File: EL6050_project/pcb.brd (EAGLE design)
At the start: 160 x 100 mm, 36 parts, among them IC1 MEGA8-P, IC2 MEGA8-P, X1 BU-SMA-V, X2 GMSTBA2

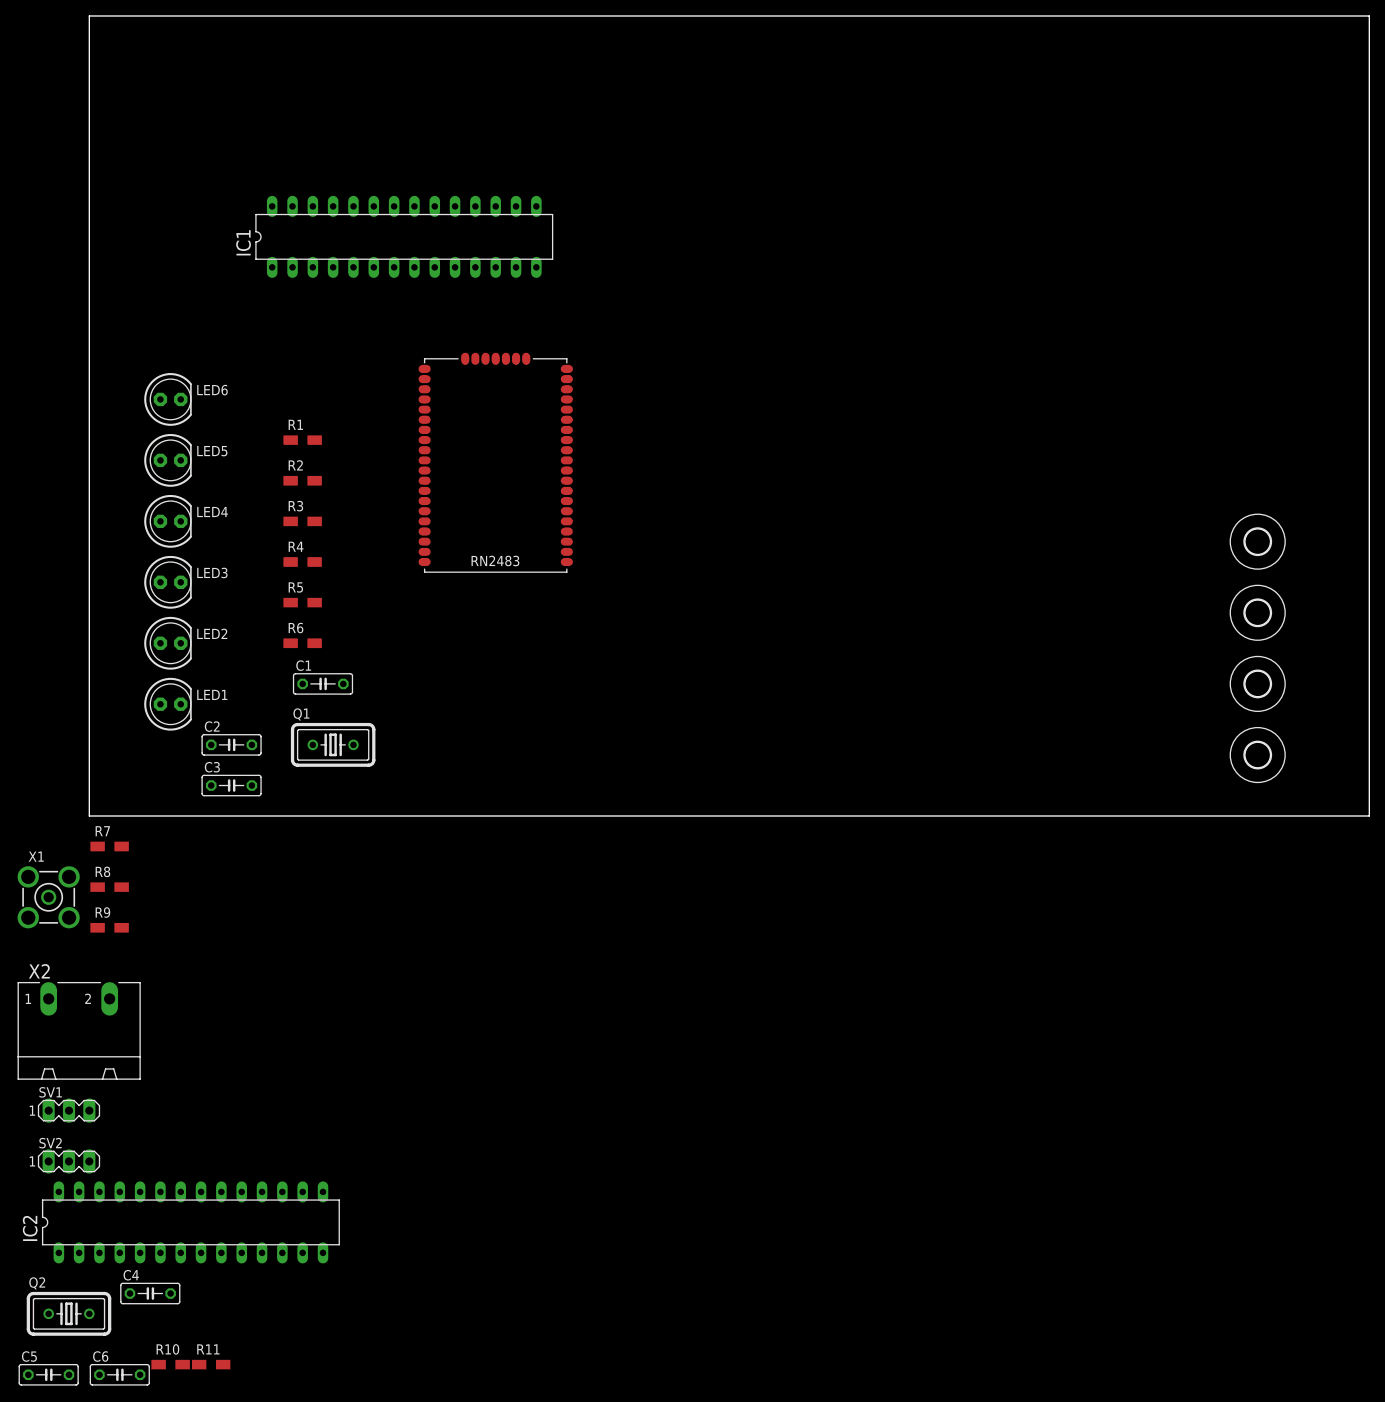
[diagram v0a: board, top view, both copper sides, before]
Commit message: all components added and board started
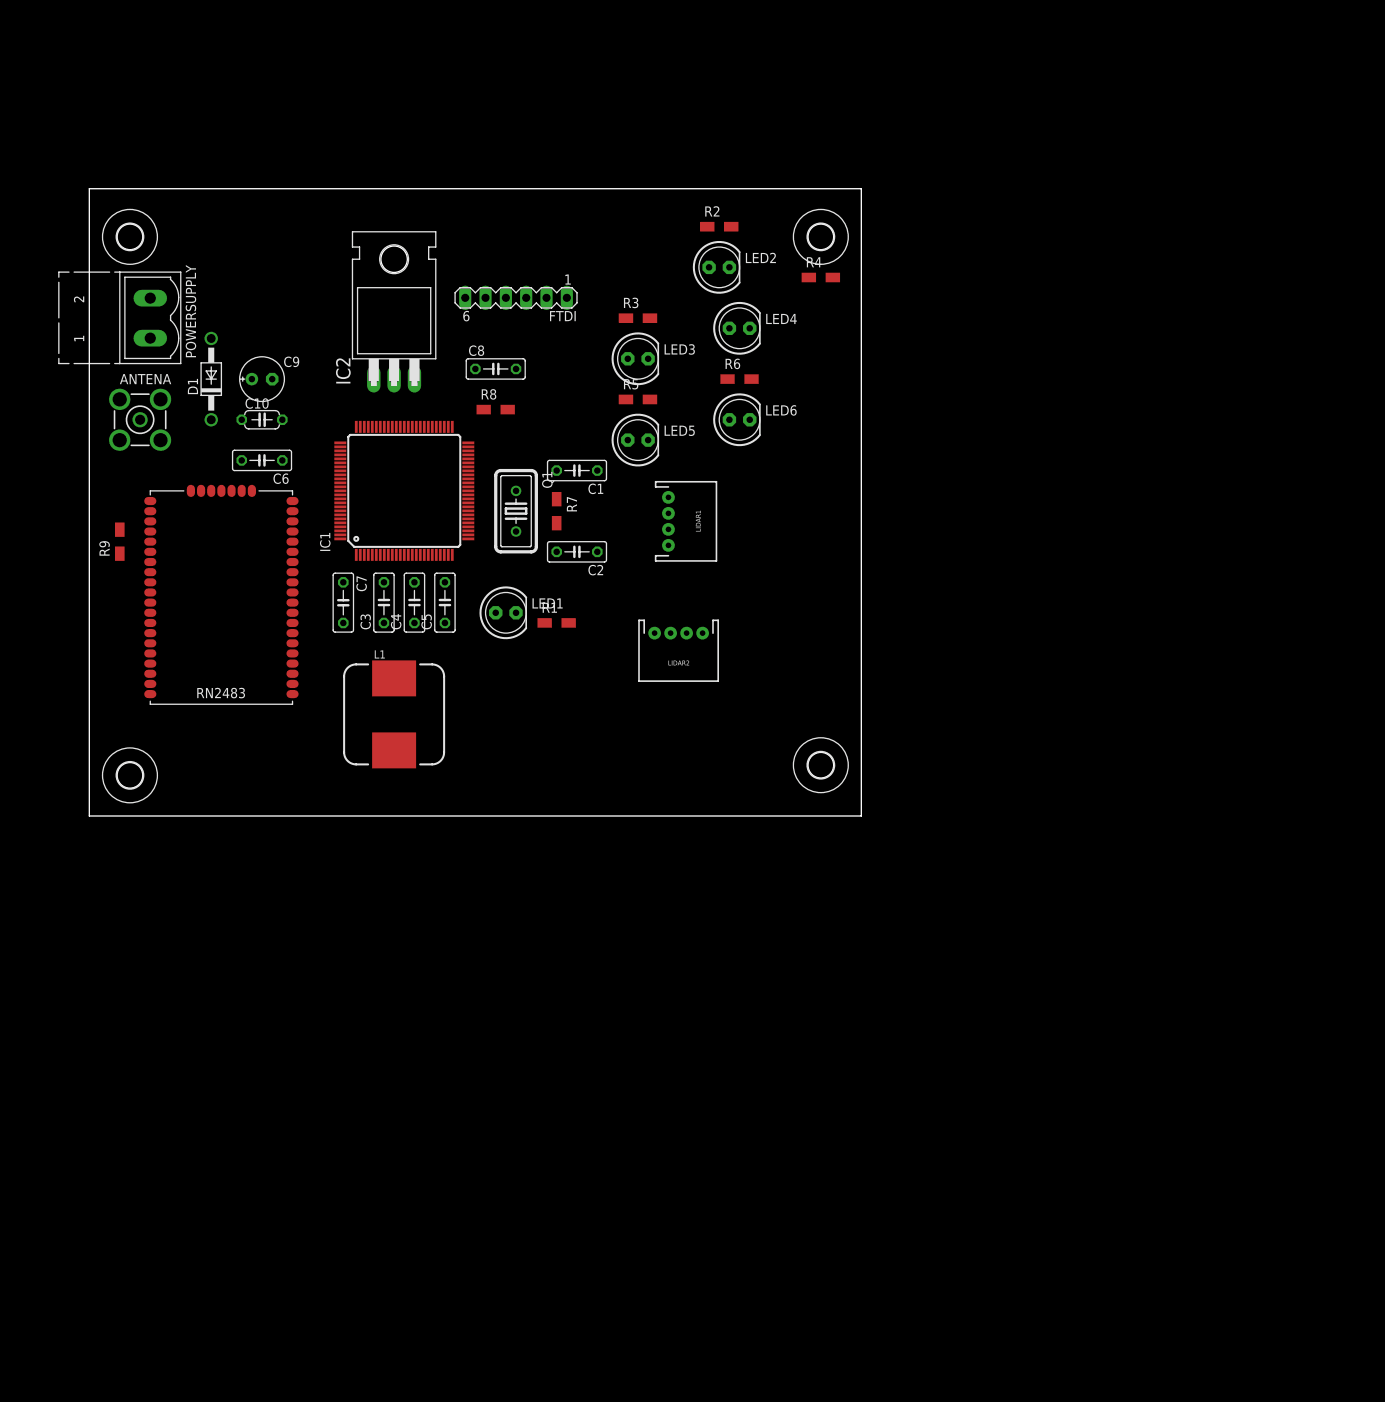
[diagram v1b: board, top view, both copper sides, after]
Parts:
- removed Q2: (no value), crystal:HC18U-V
- removed R10, R11: (no value), rcl:R1206W
- removed SV1, SV2: (no value), con-lstb:MA03-1
- removed U$1: MICROCHIP_RN2483, lora-lorawan-modules:MICROCHIP_RN2483
- removed X1: BU-SMA-V, con-coax:BU-SMA-V
- removed X2: GMSTBA2, con-phoenix-762:GMSTBA2
- added ANTENA: BU-SMA-V, con-coax:BU-SMA-V
- added C10: 100n, rcl:C050-024X044
- added C7: 100nF, rcl:C050-025X075
- added C8: 0.1u, rcl:C050-025X075
- added C9: 47u, rcl:E2,5-6E
- added D1: 1N4004, diode:DO41-10
- added FTDI: (no value), con-lstb:MA06-1
- added L1: 100mF, inductor-coilcraft2:MSS1260
- added LIDAR1, LIDAR2: (no value), sparkfun-connectors:JST-4-PTH
- added LRW-RN2903: MICROCHIP_RN2483, lora-lorawan-modules:MICROCHIP_RN2483
- added POWERSUPPLY: (no value), con-phoenix-500:MSTBV2
- C3, C4, C5, C6: value (none) -> 100nF
- IC1: value MEGA8-P -> ATMEGA2560-16AU; device atmel:DIL28-3 -> atmel-2005:TQFP100
- IC2: value MEGA8-P -> 7805T; device atmel:DIL28-3 -> linear:TO220H
- R7: value (none) -> 1M
- R8: value (none) -> 10k
- moved H2 148.6 mm to (5.08, 72.4)
- moved H1 144.0 mm to (5.08, 5.08)
- moved IC2 118.3 mm to (38.1, 64.8)
- moved C6 115.7 mm to (21.6, 44.5), turned to 180 degrees
- moved C5 108.5 mm to (44.5, 26.7), turned to 90 degrees
- moved C4 92.5 mm to (40.6, 26.7), turned to 90 degrees
- moved LED2 83.1 mm to (78.7, 68.6)
- moved H3 78.1 mm to (91.4, 72.4)
- moved R8 76.8 mm to (50.8, 50.8)
- moved LED4 75.1 mm to (81.3, 61.0)
- moved R4 73.9 mm to (91.4, 67.3)
- moved LED6 71.2 mm to (81.3, 49.5)
- moved R7 69.9 mm to (58.4, 38.1), turned to 270 degrees
- moved LED3 64.8 mm to (68.6, 57.1)
- moved R6 63.8 mm to (81.3, 54.6)
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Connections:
- removed net N$15: X2.1
- removed net N$16: R9.2, U$1.32
- removed net N$19: X2.2
- removed net N$24: IC2.4
- removed net N$26: LED1.K
- removed net N$27: LED2.K
- removed net N$28: LED3.K
- removed net N$29: LED4.K
- removed net N$30: LED5.K
- removed net N$31: LED6.K
- removed net N$35: IC2.6
- removed net N$40: IC2.12
- removed net N$43: IC1.12
- removed net N$51: IC2.14
- removed net N$58 (its old number): IC1.1, R8.1
- removed net N$61: IC2.17
- removed net N$65: IC2.18
- removed net N$66 (its old number): IC2.27
- removed net N$67: IC2.24
- removed net N$68: IC2.26
- removed net N$69 (its old number): IC2.28
- removed net N$70: IC2.5
- removed net N$71: IC2.11
- removed net N$72: IC2.13
- removed net N$73: IC2.15
- removed net N$74: IC2.16
- removed net N$75: IC2.19
- removed net N$76: IC2.1, R11.1
- removed net N$77: IC2.21
- removed net N$78: C5.2, IC2.9, Q2.2, R10.2
- removed net N$79: IC2.22
- removed net RF_LRW: U$1.23, X1.1
- removed net ULS1: SV1.3
- removed net ULS2: SV2.3
- removed net VCC: R9.1, U$1.12, U$1.34
- new net 3V3: FTDI.1, IC2.3, LRW-RN2903.12, LRW-RN2903.34, R9.1
- new net AVCC: C7.2, IC1.100, L1.1
- new net DST-CP: C8.1, FTDI.6
- new net L_DIST: IC1.40, LED6.K
- new net L_ON: IC1.42
- new net L_RED: IC1.41, LED2.K
- new net L_TRSA: IC1.39, LED3.K
- new net L_TRSB: IC1.38, LED4.K
- new net L_TRSC: IC1.37, LED5.K
- new net N$100: IC1.76
- new net N$101: IC1.78
- new net N$106: IC1.59
- new net N$107: IC1.57
- new net N$108: IC1.54
- new net N$109: IC1.53
- new net N$110: IC1.49
- new net N$111: IC1.47
- new net N$113: IC1.43
- new net N$114: IC1.8
- new net N$118: IC1.91
- new net N$119: IC1.93
- new net N$120: IC1.95
- new net N$121: IC1.97
- new net N$122: IC1.29
- new net N$123: IC1.70
- new net N$124: IC1.51
- new net N$125: IC1.55
- new net N$126: IC1.50
- new net N$127: IC1.48
- new net N$129: IC1.44
- new net N$130: IC1.9
- new net N$131: IC1.7
- new net N$134: IC1.90
- new net N$135: IC1.92
- new net N$136: IC1.94
- new net N$137: IC1.96
- new net N$138: IC1.1
- new net N$140: IC1.52
- new net N$41: C1.2, IC1.34, Q1.1, R7.1
- new net N$42: C2.2, IC1.33, Q1.2, R7.2
- new net N$46: IC1.36
- new net N$47: IC1.82
- new net N$48: IC1.84
- new net N$49: IC1.86
- new net N$50: IC1.88
- new net N$52: IC1.79
- new net N$62: IC1.73
- new net N$63: IC1.75
- new net N$84: IC1.60
- new net N$85: IC1.58
- new net N$86: IC1.56
- new net N$87: IC1.85
- new net N$88: IC1.87
- new net N$89: IC1.89
- new net N$90: IC1.69
- new net N$91: IC1.67
- new net N$92: IC1.65
- new net N$98: IC1.72
- new net N$99: IC1.74
- new net PWRIN: D1.A, POWERSUPPLY.1
- new net RF-LRW: ANTENA.1, LRW-RN2903.23
- new net RST-LRW: LRW-RN2903.32, R9.2
- new net RX-CP: FTDI.5, IC1.64
- new net RX-LID1: IC1.46, LIDAR1.2
- new net RX-LID2: IC1.13, LIDAR2.2
- new net TX-CP: FTDI.4, IC1.63
- new net TX-LID1: IC1.45, LIDAR1.1
- new net TX-LID2: IC1.12, LIDAR2.1
- net 5V: now also C10.1, C4.2, C5.2, C9.+, D1.C, FTDI.3, IC1.10, IC1.31, IC1.61, IC1.80, IC2.1, L1.2, LED1.K, LIDAR1.3, LIDAR2.3, R8.1; no longer C6.2, IC1.7, IC2.7, R11.2, R8.2, SV1.1, SV2.1
- net GND: now also ANTENA.2, ANTENA.3, ANTENA.4, ANTENA.5, C10.2, C6.2, C7.1, C9.-, FTDI.2, IC1.11, IC1.32, IC1.62, IC1.81, IC1.99, IC2.2, LIDAR1.4, LIDAR2.4, LRW-RN2903.1, LRW-RN2903.11, LRW-RN2903.20, LRW-RN2903.21, LRW-RN2903.22, LRW-RN2903.24, LRW-RN2903.26, LRW-RN2903.27, LRW-RN2903.28, LRW-RN2903.33, LRW-RN2903.41, LRW-RN2903.47, LRW-RN2903.8, POWERSUPPLY.2; no longer C6.1, IC1.8, IC2.8, SV1.2, SV2.2, U$1.1, U$1.11, U$1.20, U$1.21, U$1.22, U$1.24, U$1.26, U$1.27, U$1.28, U$1.33, U$1.41, U$1.47, U$1.8, X1.2, X1.3, X1.4, X1.5
- net N$1: now also LRW-RN2903.35; no longer U$1.35
- net N$10: now also LRW-RN2903.39; no longer U$1.39
- net N$11: now also LRW-RN2903.43; no longer U$1.43
- net N$12: now also LRW-RN2903.45; no longer U$1.45
- net N$13: now also LRW-RN2903.46; no longer U$1.46
- net N$14: now also LRW-RN2903.10; no longer U$1.10
- net N$17: now also LRW-RN2903.25; no longer U$1.25
- net N$18: now also LRW-RN2903.3; no longer U$1.3
- net N$2: now also LRW-RN2903.36; no longer U$1.36
- net N$20: now also LRW-RN2903.31; no longer U$1.31
- net N$21: now also C8.2, IC1.30, R8.2; no longer IC2.23
- net N$22: now also C6.1, IC1.98; no longer IC2.25
- net N$23: now also LRW-RN2903.2; no longer U$1.2
- net N$25: now also LRW-RN2903.30; no longer U$1.30
- net N$3: now also LRW-RN2903.37; no longer U$1.37
- net N$4: now also LRW-RN2903.38; no longer U$1.38
- net N$5: now also LRW-RN2903.40; no longer U$1.40
- net N$53: now also IC1.68; no longer IC1.11
- net N$54: now also IC1.66; no longer IC1.13
- net N$6: now also LRW-RN2903.44; no longer U$1.44
- net N$60: now also IC1.71; no longer C2.2, IC1.9, Q1.2, R7.2
- net N$64: now also IC1.77; no longer C1.2, IC1.10, Q1.1, R7.1
- net N$7: now also LRW-RN2903.14; no longer U$1.14
- net N$8: now also LRW-RN2903.13; no longer U$1.13
- net N$80: now also IC1.35; no longer IC2.20
- net N$81: now also IC1.83; no longer C4.2, IC2.10, Q2.1, R10.1
- net N$9: now also LRW-RN2903.9; no longer U$1.9
- net RX-LRW: now also IC1.3, LRW-RN2903.7; no longer IC1.2, IC2.2, U$1.6
- net TX-LRW: now also IC1.2, LRW-RN2903.6; no longer IC1.3, IC2.3, U$1.7
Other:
- board size 160 x 100 mm -> 96.5 x 78.4 mm

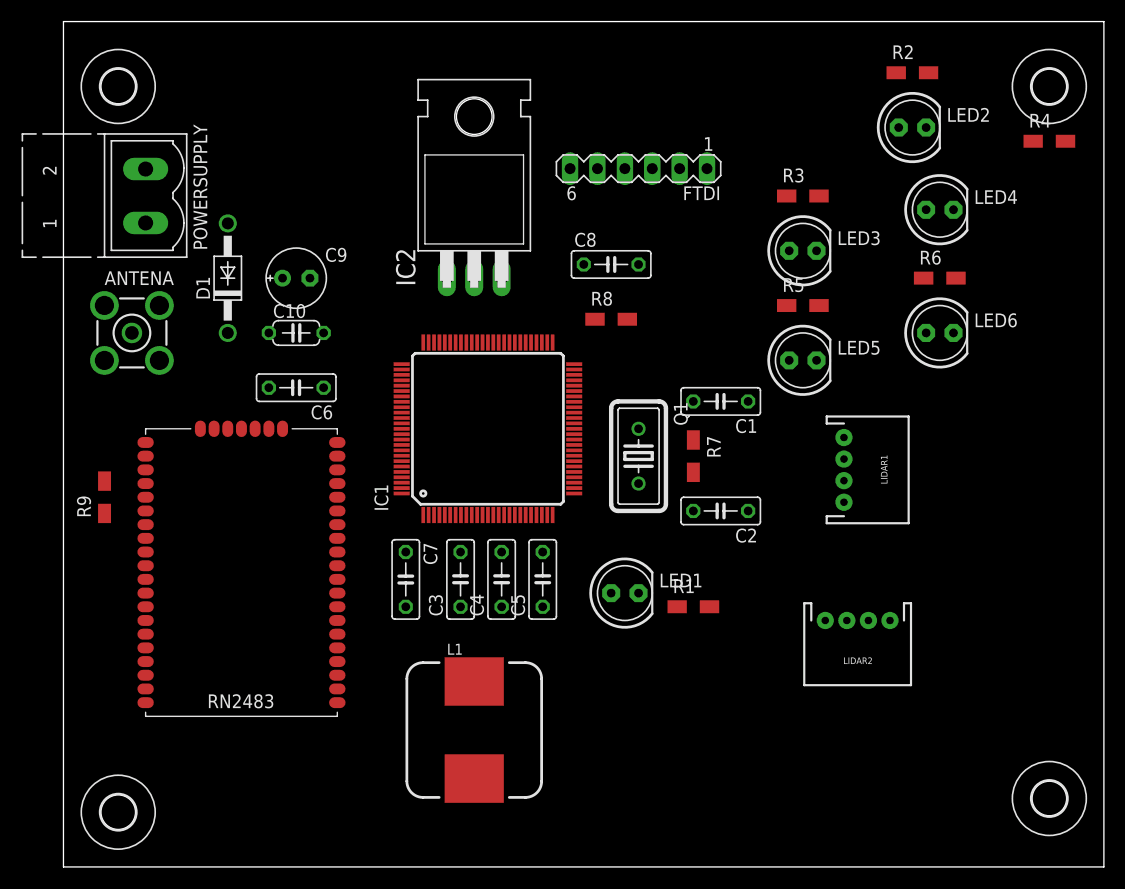
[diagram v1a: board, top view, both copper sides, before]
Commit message: end board and update schematic
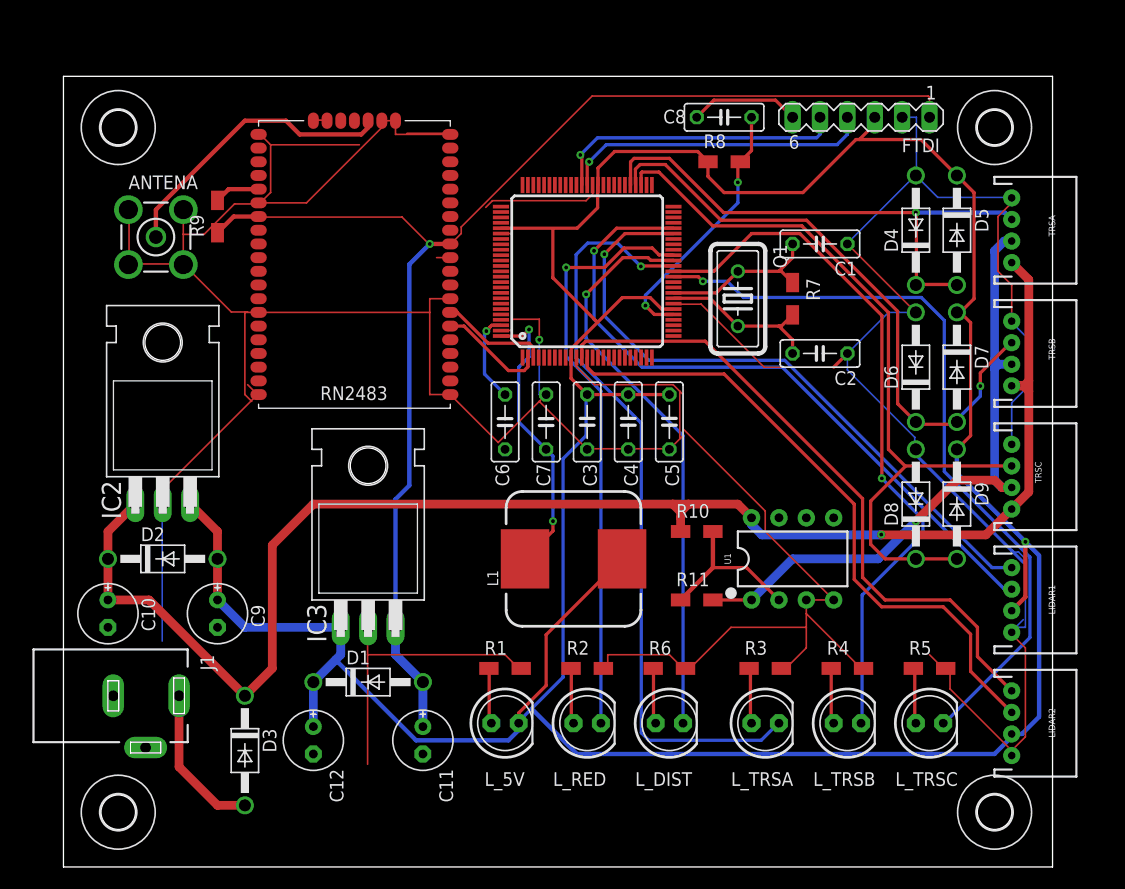
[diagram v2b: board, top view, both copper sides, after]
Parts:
- removed LED1, LED2, LED3, LED4, LED5, LED6: (no value), adafruit:LED5MM
- removed POWERSUPPLY: (no value), con-phoenix-500:MSTBV2
- added C11, C12: 10u, rcl:E2,5-6E
- added D2, D3, D4, D5, D6, D7, D8, D9: 1N4004, diode:DO41-10
- added IC3: 7805T, linear:TO220H
- added J1: DCJ0202, con-jack:DCJ0202
- added L_5V, L_DIST, L_RED, L_TRSA, L_TRSB, L_TRSC: (no value), adafruit:LED5MM
- added R10, R11: 10k, rcl:R1206W
- added TRSA, TRSB, TRSC: (no value), sparkfun-connectors:JST-4-PTH
- added U1: LM358, sparkfun-amplifiers:DIP08
- C1, C2: value (none) -> 22p
- C10: value 100n -> 47u; device rcl:C050-024X044 -> rcl:E2,5-6E
- C3, C4, C5, C6, C7: value 100nF -> 100n
- C8: value 0.1u -> 100n
- L1: value 100mF -> 10u
- Q1: value (none) -> 16MHz
- R1, R2, R3, R4, R5, R6: value (none) -> 100
- moved R2 62.9 mm to (48.6, 18.4)
- moved R4 52.4 mm to (72.7, 18.4)
- moved R6 44.0 mm to (56.2, 18.4)
- moved R3 44.0 mm to (65.1, 18.4)
- moved D1 39.7 mm to (28.3, 17.1), turned to 0 degrees
- moved IC2 35.7 mm to (9.21, 43.8)
- moved R5 35.6 mm to (80.3, 18.4)
- moved C9 32.0 mm to (14.3, 23.5), turned to 270 degrees
- moved C10 31.3 mm to (4.13, 23.5), turned to 270 degrees
- moved LRW-RN2903 30.4 mm to (18.1, 42.5)
- moved R9 28.1 mm to (14.3, 60.3)
- moved FTDI 21.2 mm to (74.0, 69.5)
- moved LIDAR1 19.7 mm to (87.9, 24.8)
- moved C6 19.6 mm to (41.0, 41.3), turned to 270 degrees
- moved C7 19.6 mm to (44.8, 41.3)
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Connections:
- net N$21 renamed RESET
- net N$41 renamed XTAL1
- net N$42 renamed XTAL2
- removed net N$108: IC1.54
- removed net N$109: IC1.53
- removed net N$125: IC1.55
- new net -15V: R11.2, TRSA.3, TRSB.3, TRSC.3, U1.1
- new net 15V: C10.+, D2.C, D3.C, IC2.1, R10.1, TRSA.4, TRSB.4, TRSC.4, U1.8
- new net N$15: R10.2, R11.1, U1.2
- new net N$16: L_TRSB.A, R4.1
- new net VO_A: D4.C, D5.A, IC1.55, TRSA.2
- new net VO_B: D6.C, D7.A, IC1.54, TRSB.2
- new net VO_C: D8.C, D9.A, IC1.53, TRSC.2
- net 3V3: now also C11.+, D1.A, IC3.3; no longer IC2.3
- net 5V: now also C12.+, D2.A, D5.C, D7.C, D9.C, IC2.3, IC3.1, L_5V.K; no longer C10.1, IC2.1, LED1.K
- net GND: now also C10.-, C11.-, C12.-, D4.A, D6.A, D8.A, IC3.2, J1.2, J1.3, TRSA.1, TRSB.1, TRSC.1, U1.3, U1.4; no longer C10.2, LED4.A, POWERSUPPLY.2, R4.1
- net L_DIST: now also L_DIST.K; no longer LED6.K
- net L_RED: now also L_RED.K; no longer LED2.K
- net L_TRSA: now also L_TRSA.K; no longer LED3.K
- net L_TRSB: now also L_TRSB.K; no longer LED4.K
- net L_TRSC: now also L_TRSC.K; no longer LED5.K
- net N$32: now also L_5V.A; no longer LED1.A
- net N$33: now also L_RED.A; no longer LED2.A
- net N$34: now also L_TRSA.A; no longer LED3.A
- net N$36: now also L_TRSC.A; no longer LED5.A
- net N$37: now also L_DIST.A; no longer LED6.A
- net PWRIN: now also D3.A, J1.1; no longer D1.A, POWERSUPPLY.1
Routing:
- net GND: track 0.00 -> 465.3 mm, vias 0 -> 1
- net 5V: track 0.00 -> 309.9 mm, vias 0 -> 1
- net 15V: track 0.00 -> 146.5 mm, vias 0 -> 1
- net 3V3: track 0.00 -> 122.8 mm, vias 0 -> 1
- net VO_C: track 0.00 -> 71.4 mm
- net L_TRSA: track 0.00 -> 71.0 mm, vias 0 -> 1
- net L_TRSC: track 0.00 -> 70.8 mm, vias 0 -> 1
- net L_TRSB: track 0.00 -> 65.8 mm, vias 0 -> 1
- net RX-LID1: track 0.00 -> 63.7 mm, vias 0 -> 1
- net TX-LID2: track 0.00 -> 60.5 mm
- net TX-LID1: track 0.00 -> 60.4 mm, vias 0 -> 1
- net -15V: track 0.00 -> 60.0 mm, vias 0 -> 1
- net RX-LID2: track 0.00 -> 59.6 mm
- net VO_B: track 0.00 -> 56.1 mm, vias 0 -> 1
- net L_RED: track 0.00 -> 54.6 mm, vias 0 -> 1
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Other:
- board size 96.5 x 78.4 mm -> 91.7 x 73.3 mm
